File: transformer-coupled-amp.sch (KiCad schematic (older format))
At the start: 47 parts, among them J1 DIN-3, Q1 МП25Б, Q2 МП25Б, Q3 МП41А, Q4 МП41А, Q5 МП40A, Q6 П213Б, Q7 П213Б, T1 Transformer_1P_1S

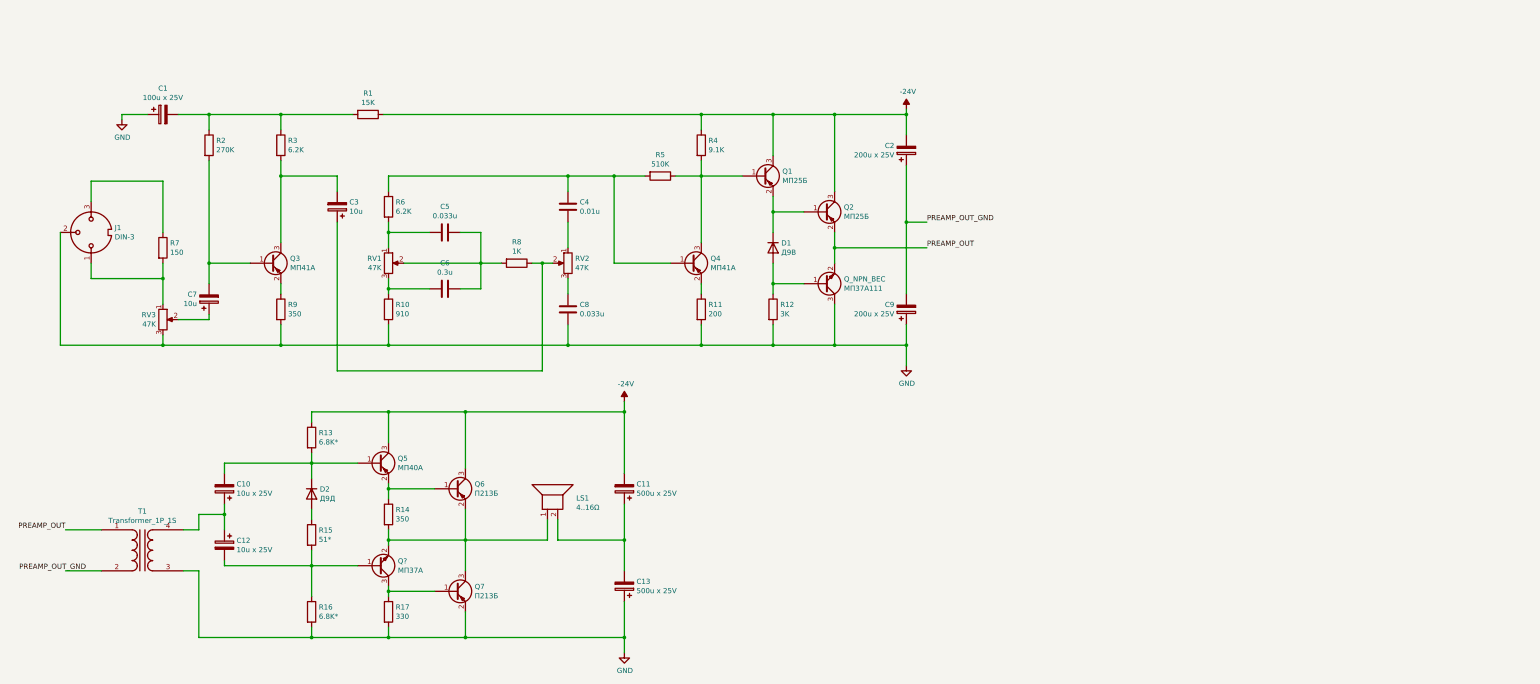
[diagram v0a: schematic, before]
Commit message: Finish drawing schematics
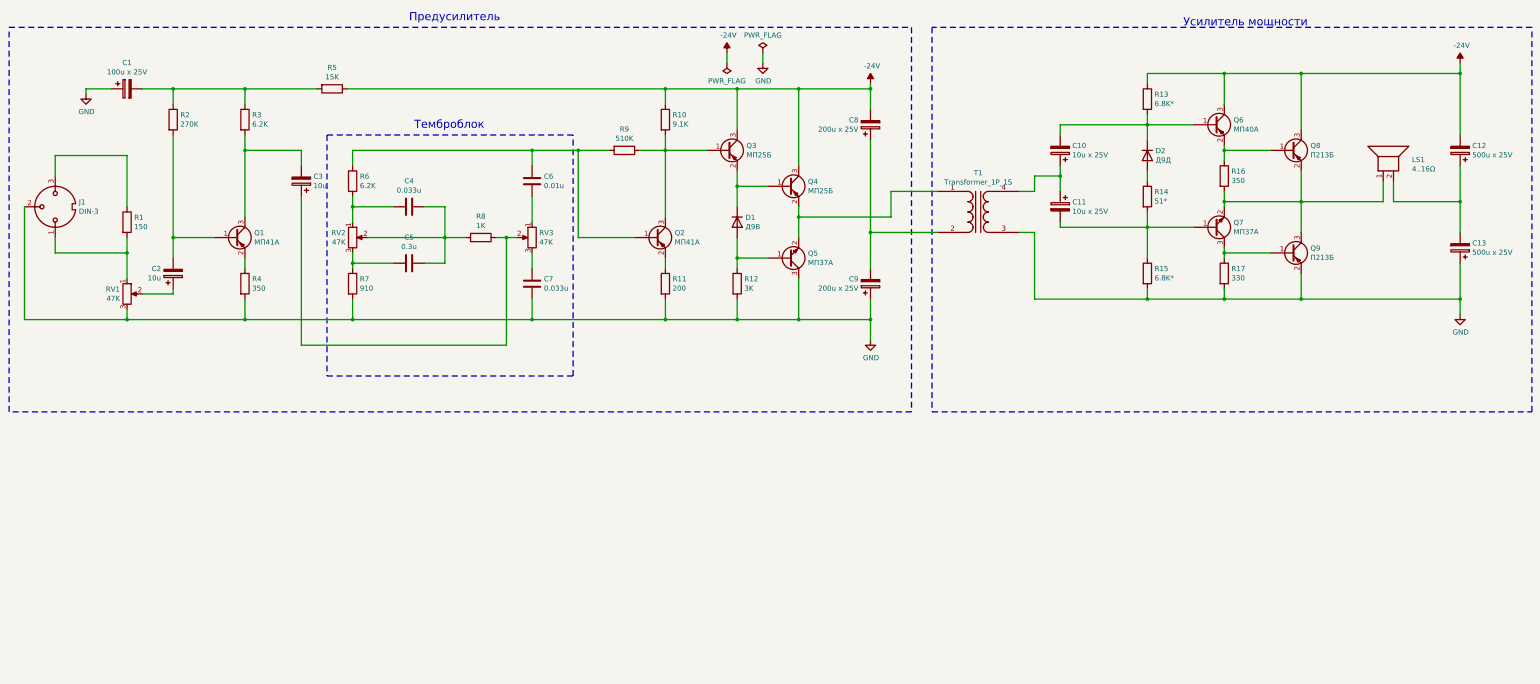
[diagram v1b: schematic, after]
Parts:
- removed МП37А: Q?, symbol Device:Q_NPN_BEC
- removed МП37А111: Q_NPN_BEC, symbol Device:Q_NPN_BEC
- added Q5, Q7: МП37А, symbol Device:Q_NPN_BEC
- renumbered C12 to C11, C11 to C12, C7 to C2, C5 to C4, C6 to C5, C4 to C6, C8 to C7, C2 to C8, Q3 to Q1, Q4 to Q2, Q1 to Q3, Q2 to Q4, Q5 to Q6, Q6 to Q8, Q7 to Q9, R7 to R1, R4 to R10, R15 to R14, R16 to R15, R14 to R16, R9 to R4, R1 to R5, R10 to R7, R5 to R9, RV3 to RV1, RV1 to RV2, RV2 to RV3
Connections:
- net GND: now also Q5.3 (C)
- net at C11.2, R14.2, R15.1: now also Q7.1 (B)
- net at D1.2 (A), R12.1: now also Q5.1 (B)
- net at LS1.1, Q8.2 (E), Q9.3 (C)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: now also Q7.2 (E)
- net at Q9.1 (B), R17.1: now also Q7.3 (C)
- net PREAMP_OUT: no longer names the net of Q4.2 (E), T1.1 (AA)
- net PREAMP_OUT: now also Q5.2 (E)
- net PREAMP_OUT_GND: no longer names the net of C8.1, C9.2, T1.2 (AB)
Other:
- note added: "Предусилитель"
- note added: "Темброблок"
- note added: "Усилитель мощности"
- moved on the sheet: C1, C10, C11, C12, C13, C2, C3, C4, C5, C6, C7, C8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
